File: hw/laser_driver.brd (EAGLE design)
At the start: 38.1 x 12.7 mm, 10 parts, among them IC1 895-FT232RL, IC2 998-MIC5209-3.0YM, X1 798-ZX62RD-AB-5P8

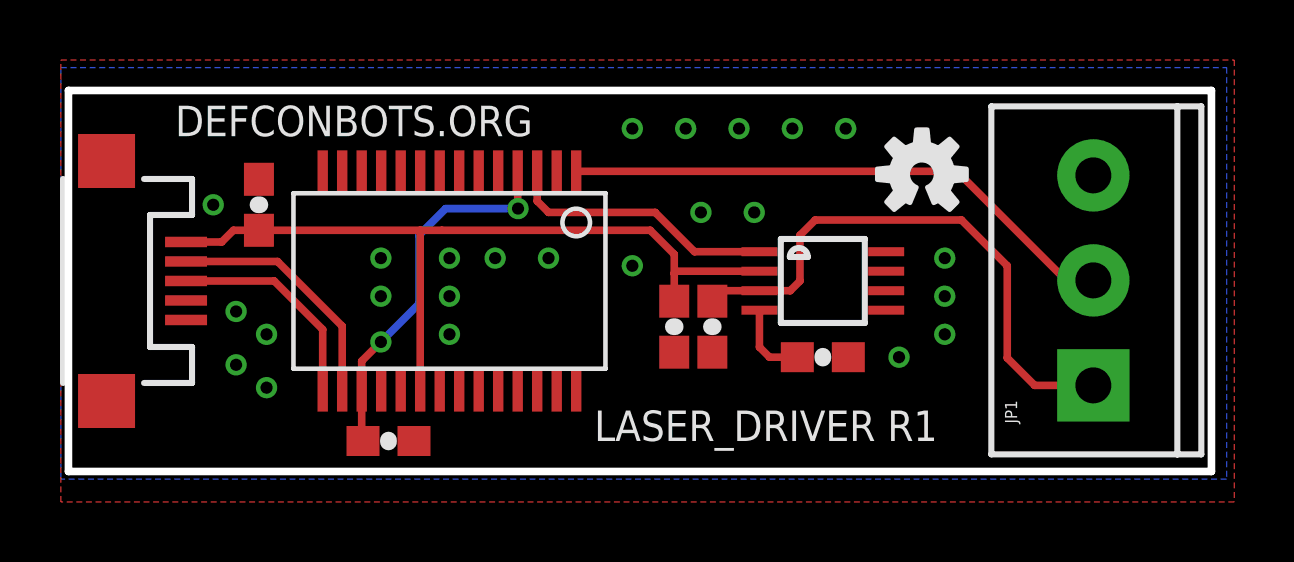
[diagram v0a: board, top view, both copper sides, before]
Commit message: Cleanup for fab. Add bom and gerbers.
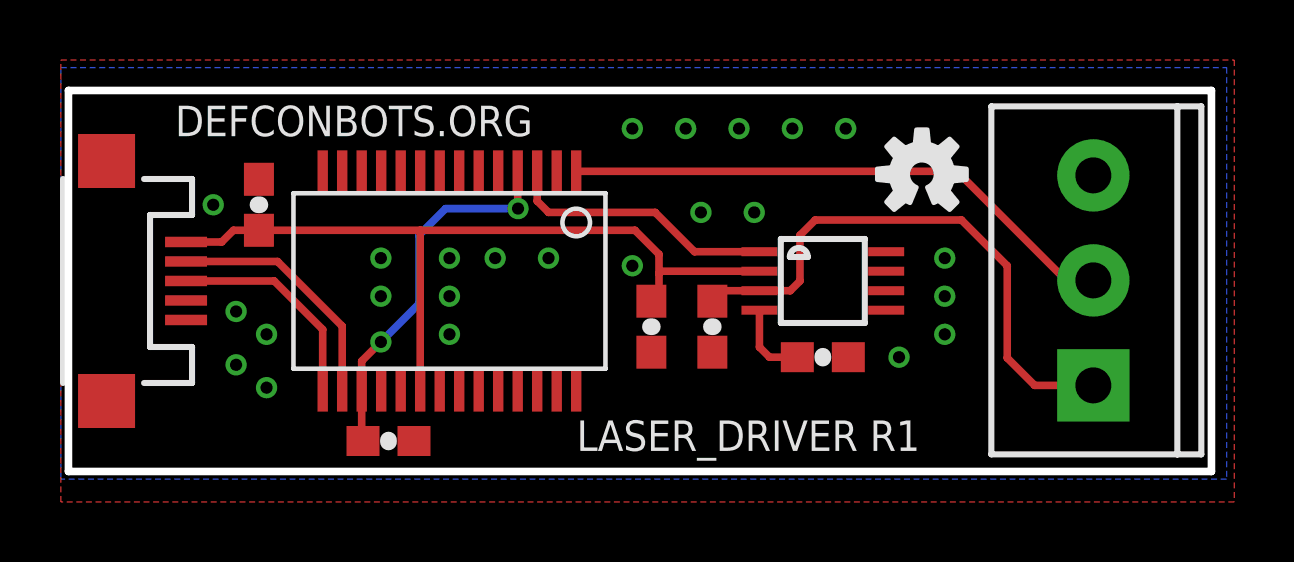
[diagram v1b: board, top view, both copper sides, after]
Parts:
- moved C3 0.76 mm to (19.4, 4.83)
